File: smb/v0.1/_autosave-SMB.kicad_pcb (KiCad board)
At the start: 2 copper layers, 83 parts, among them IC101 ATMEGA1284-A, J102 RTS_RESET, J103 ICSP, J104 SERIAL_REV, J202 USD_CONN, J401 HR911105_RJ45, P1 CONN_2, P101 I2C_CONN, P102 CONN_6, P103 CONN_5X2, P104 CONN_5X2, P301 CONN_2, SW101-RESET SKQGAKE010, U201 ENC28J60, U202 LM1117IMP-3.3, U203 74LVC1G126GW, U204 74LVC1G126GW, U205 74LVC1G126GW, U206 74LVC1G126GW, U301 74HC08, U302 MP2562DS, X101 16MHz, X201 25MHz

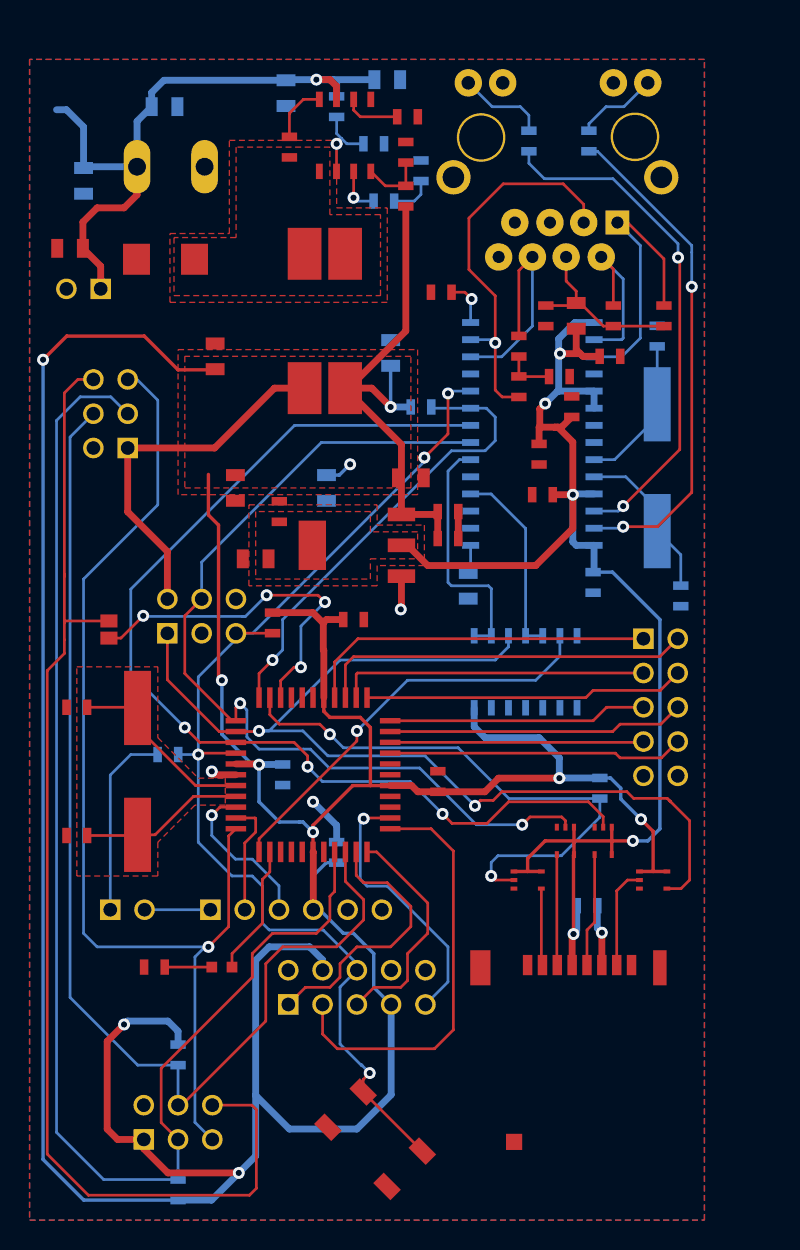
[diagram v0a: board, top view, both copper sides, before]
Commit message: modif schema
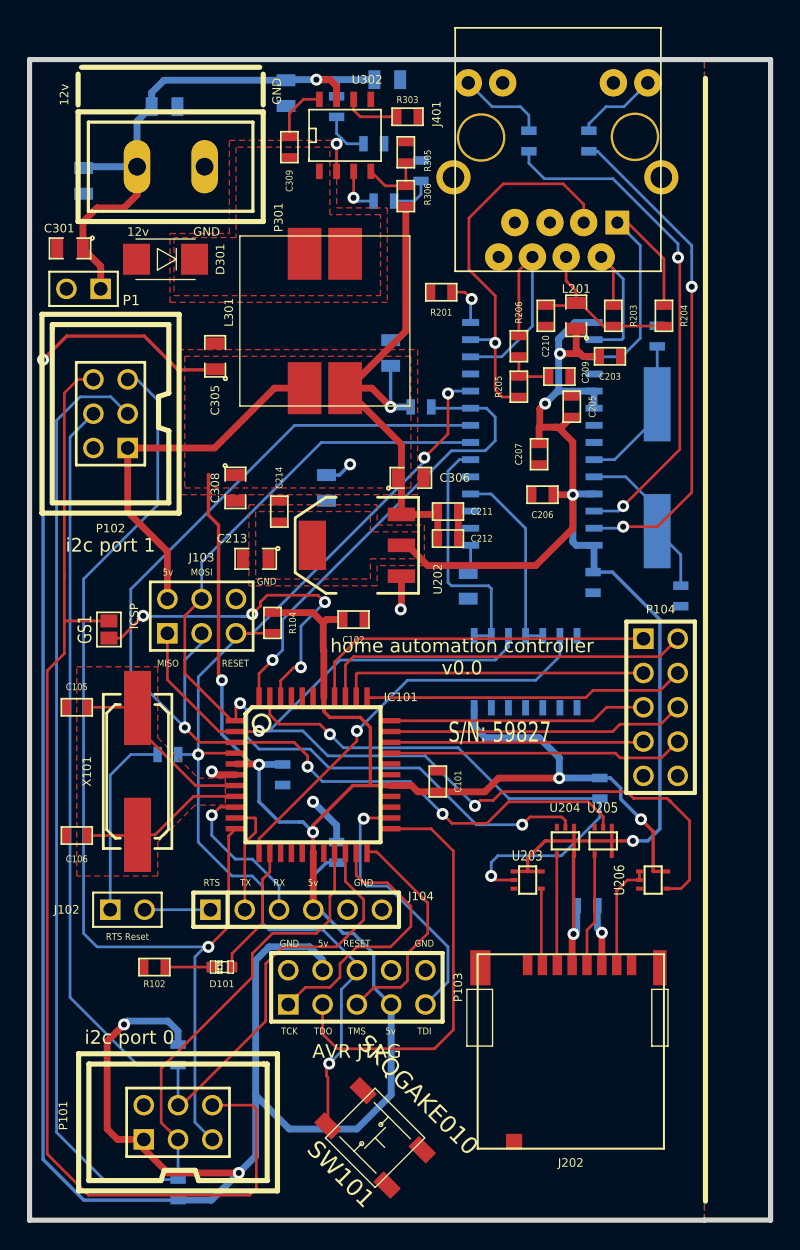
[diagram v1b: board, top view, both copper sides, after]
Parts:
- removed SW101-RESET: SKQGAKE010, SKQGAKE010
- removed logo_xplduino (x2): VAL**, logo_xplduino
- added SW101: SKQGAKE010, SKQGAKE010, F.Cu at (75.6, 179.9)
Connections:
- J103 pad 3: (no net) -> SPI_CLK
- U206 pad 1: +5V -> MISO_33
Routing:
- net SPI_CLK: track 78.4 -> 85.9 mm
- net +12V: track 50.1 -> 44.5 mm
- net /RESET: track 85.0 -> 80.6 mm
- net +5V: track 346.8 -> 345.8 mm
- net MISO_33: track 7.51 -> 8.15 mm
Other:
- board outline added: 54.9 x 86 mm
